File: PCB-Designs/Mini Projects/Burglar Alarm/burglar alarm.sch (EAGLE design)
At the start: 8 parts, among them Q1 BC557, T1 BC547

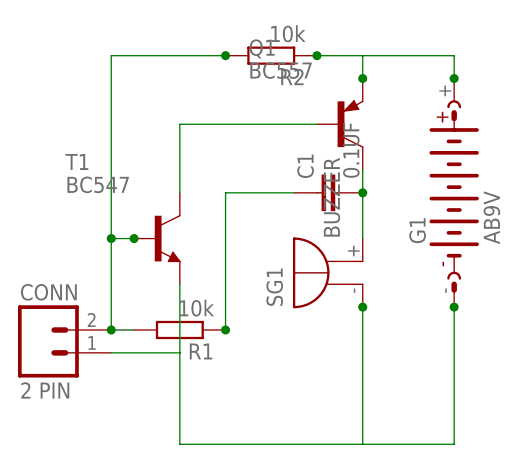
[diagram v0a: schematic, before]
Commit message: bulgral alarm...
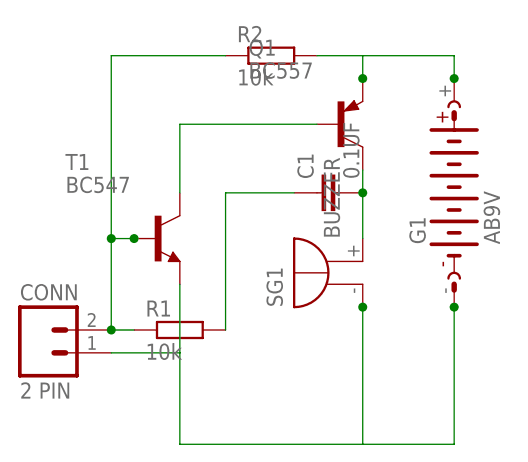
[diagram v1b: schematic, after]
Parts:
- R1, R2: device resistor:R-EU_0204/5 -> rcl:R-EU_0204/7
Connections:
- net N$2: now also R1.2; no longer R1.1
- net N$4: now also R1.1, R2.1; no longer R1.2, R2.2
- net N$5: now also R2.2; no longer R2.1
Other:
- moved on the sheet: R1, R2
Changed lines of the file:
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@@
 <?xml version="1.0" encoding="utf-8"?>
 <!DOCTYPE eagle SYSTEM "eagle.dtd">
-<eagle version="6.5.0">
+<eagle version="6.1">
 <drawing>
 <settings>
@@
 <part name="Q1" library="transistor-pnp" deviceset="BC557" device=""/>
 <part name="C1" library="capacitor-wima" deviceset="C" device="2.5/2" value="0.1UF"/>
-<part name="R1" library="resistor" deviceset="R-EU_" device="0204/5" value="10k"/>
-<part name="R2" library="resistor" deviceset="R-EU_" device="0204/5" value="10k"/>
 <part name="G1" library="battery" deviceset="AB9V" device=""/>
 <part name="SG1" library="buzzer" deviceset="F/QMB" device="" value="BUZZER"/>
 <part name="CONN" library="con-amp-quick" deviceset="M02" device="" value="2 PIN"/>
+<part name="R1" library="rcl" deviceset="R-EU_" device="0204/7" value="10k"/>
+<part name="R2" library="rcl" deviceset="R-EU_" device="0204/7" value="10k"/>
 </parts>
 <sheets>
@@
 <instance part="Q1" gate="G$1" x="48.26" y="66.04"/>
 <instance part="C1" gate="G$1" x="45.72" y="58.42" rot="R90"/>
-<instance part="R1" gate="G$1" x="30.48" y="43.18" rot="R180"/>
-<instance part="R2" gate="G$1" x="40.64" y="73.66" rot="R180"/>
 <instance part="G1" gate="G$1" x="60.96" y="58.42" rot="R90"/>
 <instance part="SG1" gate="G$1" x="48.26" y="48.26" rot="R90"/>
 <instance part="CONN" gate="G$1" x="15.24" y="40.64"/>
+<instance part="R1" gate="G$1" x="30.48" y="43.18"/>
+<instance part="R2" gate="G$1" x="40.64" y="73.66"/>
 </instances>
 <busses>
@@
 <segment>
 <pinref part="C1" gate="G$1" pin="1"/>
-<pinref part="R1" gate="G$1" pin="1"/>
 <wire x1="43.18" y1="58.42" x2="35.56" y2="58.42" width="0.1524" layer="91"/>
 <wire x1="35.56" y1="58.42" x2="35.56" y2="43.18" width="0.1524" layer="91"/>
-<junction x="35.56" y="43.18"/>
+<pinref part="R1" gate="G$1" pin="2"/>
 </segment>
 </net>
@@
 <wire x1="25.4" y1="53.34" x2="22.86" y2="53.34" width="0.1524" layer="91"/>
 <wire x1="22.86" y1="53.34" x2="22.86" y2="43.18" width="0.1524" layer="91"/>
-<pinref part="R1" gate="G$1" pin="2"/>
 <wire x1="22.86" y1="43.18" x2="25.4" y2="43.18" width="0.1524" layer="91"/>
 <wire x1="22.86" y1="53.34" x2="22.86" y2="73.66" width="0.1524" layer="91"/>
 <wire x1="22.86" y1="73.66" x2="35.56" y2="73.66" width="0.1524" layer="91"/>
-<pinref part="R2" gate="G$1" pin="2"/>
 <junction x="25.4" y="53.34"/>
 <junction x="22.86" y="43.18"/>
-<junction x="35.56" y="73.66"/>
 <junction x="22.86" y="53.34"/>
 <pinref part="CONN" gate="G$1" pin="2"/>
+<pinref part="R1" gate="G$1" pin="1"/>
+<pinref part="R2" gate="G$1" pin="1"/>
 </segment>
 </net>
@@
 <wire x1="60.96" y1="73.66" x2="50.8" y2="73.66" width="0.1524" layer="91"/>
 <wire x1="45.72" y1="73.66" x2="50.8" y2="73.66" width="0.1524" layer="91"/>
-<pinref part="R2" gate="G$1" pin="1"/>
 <junction x="50.8" y="71.12"/>
 <junction x="60.96" y="71.12"/>
-<junction x="45.72" y="73.66"/>
+<pinref part="R2" gate="G$1" pin="2"/>
 </segment>
 </net>
